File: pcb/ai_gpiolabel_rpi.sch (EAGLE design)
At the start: 3 parts

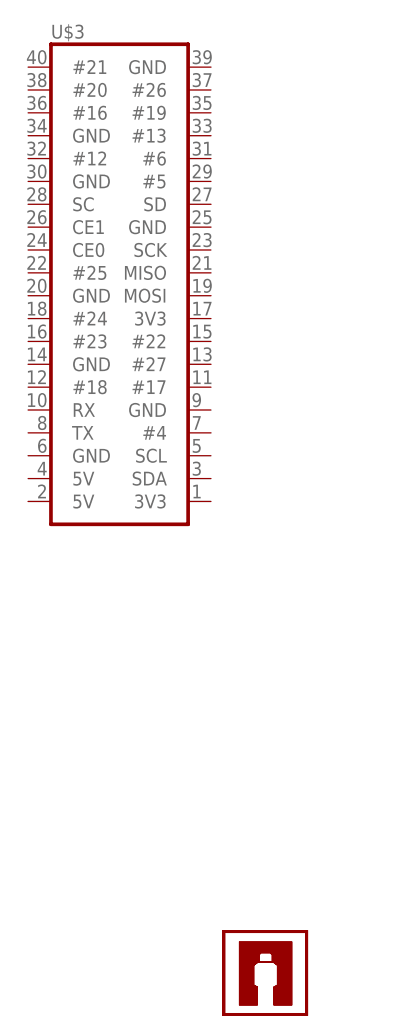
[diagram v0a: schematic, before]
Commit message: updating
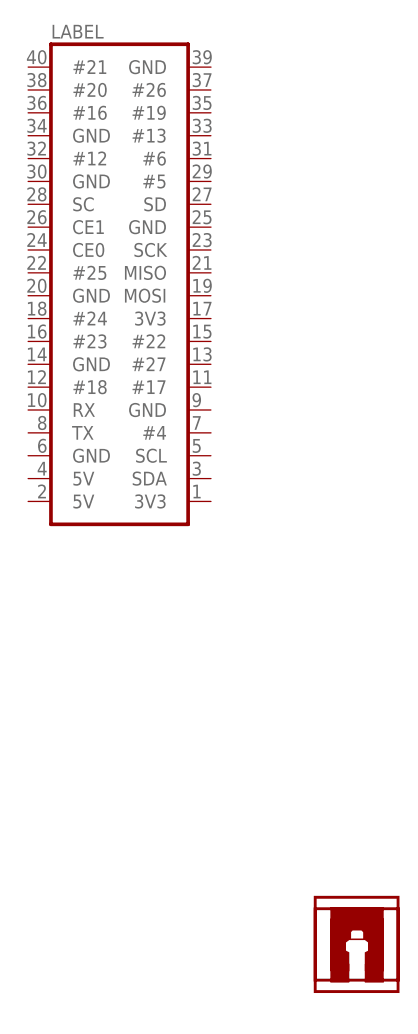
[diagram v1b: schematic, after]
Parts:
- renumbered U$3 to LABEL
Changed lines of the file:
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@@
 <grid distance="50" unitdist="mil" unit="mil" style="lines" multiple="1" display="yes" altdistance="0.01" altunitdist="inch" altunit="inch"/>
 <layers>
-<layer number="1" name="Top" color="4" fill="1" visible="yes" active="no"/>
-<layer number="16" name="Bottom" color="1" fill="1" visible="yes" active="no"/>
-<layer number="17" name="Pads" color="2" fill="1" visible="yes" active="no"/>
-<layer number="18" name="Vias" color="2" fill="1" visible="yes" active="no"/>
-<layer number="19" name="Unrouted" color="6" fill="1" visible="yes" active="no"/>
-<layer number="20" name="Dimension" color="15" fill="1" visible="yes" active="no"/>
-<layer number="21" name="tPlace" color="7" fill="1" visible="yes" active="no"/>
-<layer number="22" name="bPlace" color="7" fill="1" visible="yes" active="no"/>
-<layer number="23" name="tOrigins" color="15" fill="1" visible="yes" active="no"/>
-<layer number="24" name="bOrigins" color="15" fill="1" visible="yes" active="no"/>
-<layer number="25" name="tNames" color="7" fill="1" visible="yes" active="no"/>
-<layer number="26" name="bNames" color="7" fill="1" visible="yes" active="no"/>
-<layer number="27" name="tValues" color="7" fill="1" visible="yes" active="no"/>
-<layer number="28" name="bValues" color="7" fill="1" visible="yes" active="no"/>
+<layer number="1" name="Top" color="4" fill="1" visible="no" active="no"/>
+<layer number="16" name="Bottom" color="1" fill="1" visible="no" active="no"/>
+<layer number="17" name="Pads" color="2" fill="1" visible="no" active="no"/>
+<layer number="18" name="Vias" color="2" fill="1" visible="no" active="no"/>
+<layer number="19" name="Unrouted" color="6" fill="1" visible="no" active="no"/>
+<layer number="20" name="Dimension" color="15" fill="1" visible="no" active="no"/>
+<layer number="21" name="tPlace" color="7" fill="1" visible="no" active="no"/>
+<layer number="22" name="bPlace" color="7" fill="1" visible="no" active="no"/>
+<layer number="23" name="tOrigins" color="15" fill="1" visible="no" active="no"/>
+<layer number="24" name="bOrigins" color="15" fill="1" visible="no" active="no"/>
+<layer number="25" name="tNames" color="7" fill="1" visible="no" active="no"/>
+<layer number="26" name="bNames" color="7" fill="1" visible="no" active="no"/>
+<layer number="27" name="tValues" color="7" fill="1" visible="no" active="no"/>
+<layer number="28" name="bValues" color="7" fill="1" visible="no" active="no"/>
 <layer number="29" name="tStop" color="7" fill="3" visible="no" active="no"/>
 <layer number="30" name="bStop" color="7" fill="6" visible="no" active="no"/>
@@
 <layer number="35" name="tGlue" color="7" fill="4" visible="no" active="no"/>
 <layer number="36" name="bGlue" color="7" fill="5" visible="no" active="no"/>
-<layer number="37" name="tTest" color="7" fill="1" visible="yes" active="no"/>
-<layer number="38" name="bTest" color="7" fill="1" visible="yes" active="no"/>
+<layer number="37" name="tTest" color="7" fill="1" visible="no" active="no"/>
+<layer number="38" name="bTest" color="7" fill="1" visible="no" active="no"/>
 <layer number="39" name="tKeepout" color="4" fill="11" visible="no" active="no"/>
 <layer number="40" name="bKeepout" color="1" fill="11" visible="no" active="no"/>
@@
 <layer number="44" name="Drills" color="7" fill="1" visible="no" active="no"/>
 <layer number="45" name="Holes" color="7" fill="1" visible="no" active="no"/>
-<layer number="46" name="Milling" color="3" fill="1" visible="yes" active="no"/>
-<layer number="47" name="Measures" color="7" fill="1" visible="yes" active="no"/>
-<layer number="48" name="Document" color="7" fill="1" visible="yes" active="no"/>
-<layer number="49" name="Reference" color="7" fill="1" visible="yes" active="no"/>
-<layer number="50" name="dxf" color="7" fill="1" visible="yes" active="no"/>
-<layer number="51" name="tDocu" color="7" fill="1" visible="yes" active="no"/>
-<layer number="52" name="bDocu" color="7" fill="1" visible="yes" active="no"/>
-<layer number="53" name="tGND_GNDA" color="7" fill="9" visible="yes" active="no"/>
-<layer number="54" name="bGND_GNDA" color="1" fill="9" visible="yes" active="no"/>
-<layer number="56" name="wert" color="7" fill="1" visible="yes" active="no"/>
-<layer number="57" name="tCAD" color="7" fill="1" visible="yes" active="no"/>
+<layer number="46" name="Milling" color="3" fill="1" visible="no" active="no"/>
+<layer number="47" name="Measures" color="7" fill="1" visible="no" active="no"/>
+<layer number="48" name="Document" color="7" fill="1" visible="no" active="no"/>
+<layer number="49" name="Reference" color="7" fill="1" visible="no" active="no"/>
+<layer number="50" name="dxf" color="7" fill="1" visible="no" active="no"/>
+<layer number="51" name="tDocu" color="7" fill="1" visible="no" active="no"/>
+<layer number="52" name="bDocu" color="7" fill="1" visible="no" active="no"/>
+<layer number="53" name="tGND_GNDA" color="7" fill="9" visible="no" active="no"/>
+<layer number="54" name="bGND_GNDA" color="1" fill="9" visible="no" active="no"/>
+<layer number="56" name="wert" color="7" fill="1" visible="no" active="no"/>
+<layer number="57" name="tCAD" color="7" fill="1" visible="no" active="no"/>
 <layer number="90" name="Modules" color="5" fill="1" visible="yes" active="yes"/>
 <layer number="91" name="Nets" color="2" fill="1" visible="yes" active="yes"/>
@@
 <layer number="97" name="Info" color="7" fill="1" visible="yes" active="yes"/>
 <layer number="98" name="Guide" color="6" fill="1" visible="yes" active="yes"/>
+<layer number="99" name="SpiceOrder" color="7" fill="1" visible="no" active="no"/>
 <layer number="100" name="Muster" color="7" fill="1" visible="no" active="no"/>
 <layer number="101" name="Patch_Top" color="12" fill="4" visible="no" active="yes"/>
@@
 </part>
 <part name="U$2" library="Ai_Miscellany" deviceset="AI-LOGO" device="XS"/>
-<part name="U$3" library="Ai_Connectors" deviceset="2X20-RPI" device="-NOFIRST" value="2X20-RPI-NOFIRST"/>
+<part name="LABEL" library="Ai_Connectors" deviceset="2X20-RPI" device="-NOFIRST" value="2X20-RPI-NOFIRST"/>
 <part name="U$4" library="Ai_Miscellany" deviceset="AI-LOGO" device="XS"/>
 </parts>
@@
 <instances>
 <instance part="FRAME1" gate="G$1" x="0" y="0"/>
-<instance part="FRAME1" gate="G$2" x="147.32" y="0"/>
-<instance part="U$2" gate="G$1" x="134.62" y="13.97"/>
-<instance part="U$3" gate="G$1" x="123.19" y="95.25"/>
-<instance part="U$4" gate="G$1" x="134.62" y="13.97"/>
+<instance part="FRAME1" gate="G$2" x="154.94" y="3.81"/>
+<instance part="U$2" gate="G$1" x="144.78" y="17.78"/>
+<instance part="LABEL" gate="G$1" x="123.19" y="95.25"/>
+<instance part="U$4" gate="G$1" x="144.78" y="16.51"/>
 </instances>
 <busses>
